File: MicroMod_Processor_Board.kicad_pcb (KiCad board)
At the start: 4 copper layers, 22 x 22 mm, 4 parts, among them J1 MICROMOD-2222

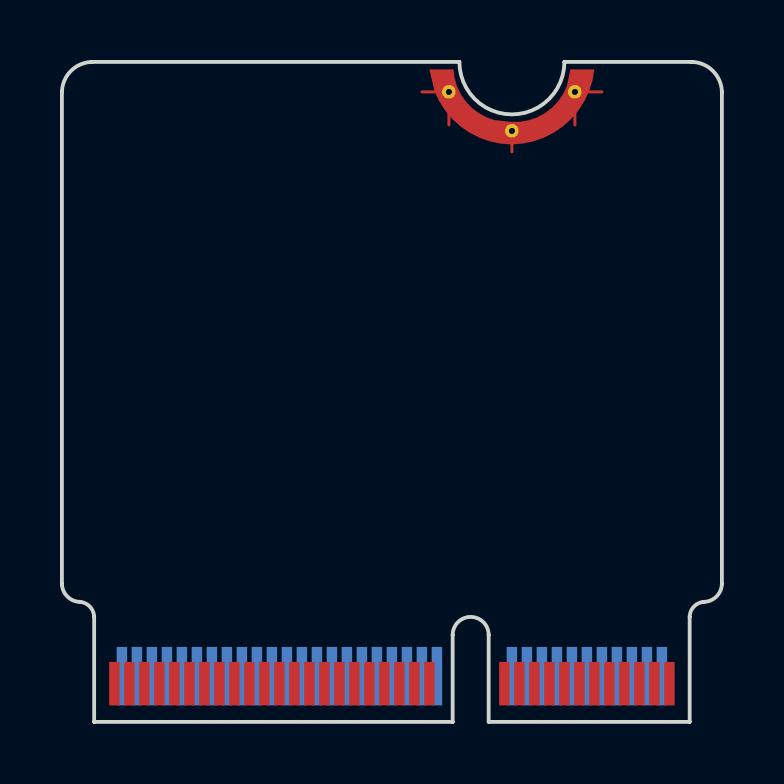
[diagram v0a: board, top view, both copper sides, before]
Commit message: Add files via upload
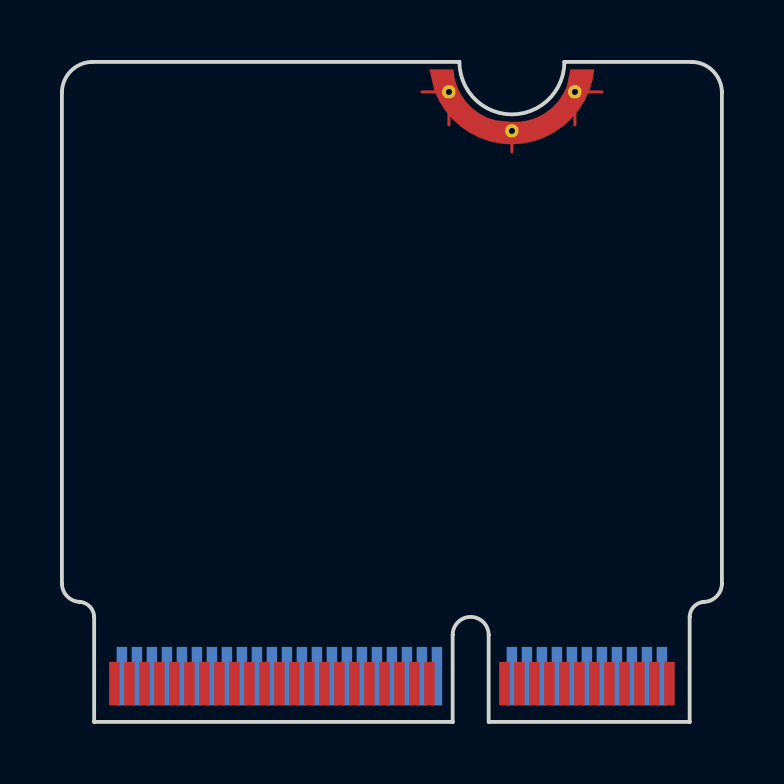
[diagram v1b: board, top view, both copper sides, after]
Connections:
- net /0-~BOOT~ renamed /0-~{BOOT}
- net /4-I2C_~INT renamed /4-I2C_~{INT}
- net /5-~CS renamed /5-~{CS}
- net /~RESET renamed /~{RESET}
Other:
- net class Default removed
